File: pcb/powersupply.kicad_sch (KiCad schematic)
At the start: 33 parts, among them Q2 AO3401A, Q3 2N7002, Q9 AO3401A, U10 SMAJ16A-TR, U4 TPS54302, U5 SMAJ16A-TR, U6 AMS1117-3.3

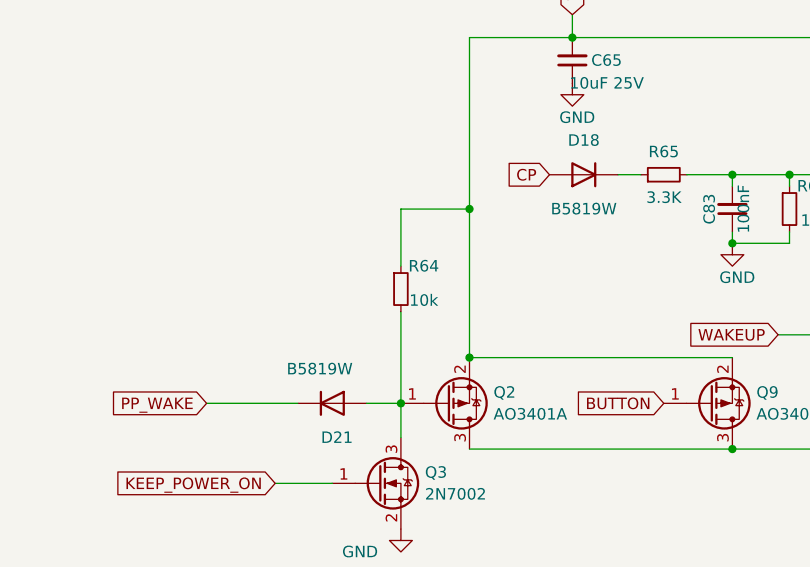
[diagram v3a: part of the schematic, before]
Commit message: Made PP standby and button pullup 1k Improved connection of TVS diode
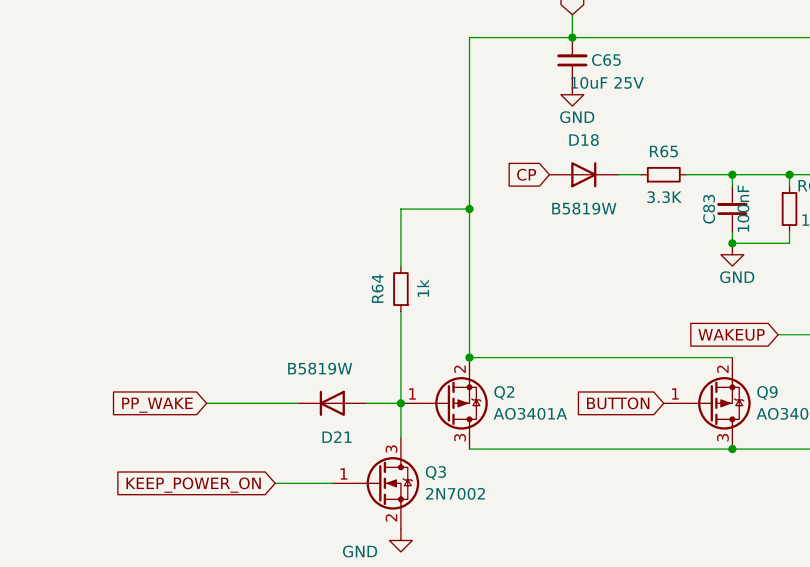
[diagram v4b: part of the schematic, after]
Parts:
- R64: value 10k -> 1k; LCSC C17414 -> C17513; LINK https://jlcpcb.com/partdetail/18102-0805W8F1002T5E/C17414 -> https://jlcpcb.com/partdetail/18201-0805W8F1001T5E/C17513
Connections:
- net 12V_P: now also R64.2; no longer R64.1
- net at D21.2 (A), Q2.1 (G), Q3.3 (D): now also R64.1; no longer R64.2
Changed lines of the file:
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@@
+    )
+  )
+  (symbol (lib_id "Device:R_Small") (at 109.22 72.39 180) (unit 1)
+    (in_bom yes) (on_board yes) (dnp no)
+    (property "Reference" "R64" (at 106.68 72.39 90)
+      (effects (font (size 1.27 1.27)))
+    )
+    (property "Value" "1k" (at 111.76 72.39 90)
+      (effects (font (size 1.27 1.27)))
+    )
+    (property "Footprint" "Resistor_SMD:R_0805_2012Metric_Pad1.20x1.40mm_HandSolder" (at 109.22 72.39 0)
+      (effects (font (size 1.27 1.27)) hide)
+    )
+    (property "Datasheet" "https://datasheet.lcsc.com/lcsc/1811101920_UNI-ROYAL-Uniroyal-Elec-0603WAF3301T5E_C22978.pdf" (at 109.22 72.39 0)
+      (effects (font (size 1.27 1.27)) hide)
+    )
+    (property "LCSC" "C17513" (at 109.22 72.39 90)
+      (effects (font (size 1.27 1.27)) hide)
+    )
+    (property "LINK" "https://jlcpcb.com/partdetail/18201-0805W8F1001T5E/C17513" (at 109.22 72.39 0)
+      (effects (font (size 1.27 1.27)) hide)
+    )
+    (pin "1")
+    (pin "2")
+    (instances
+      (project "qca7000"
+        (path "/e63e39d7-6ac0-4ffd-8aa3-1841a4541b55/81db238c-e53f-4d52-98ea-36a1df697651"
+          (reference "R64") (unit 1)
+        )
+      )
     )
   )
@@
         )
       )
-    )
-  )
-  (symbol (lib_id "Device:R_Small") (at 109.22 72.39 0) (unit 1)
-    (in_bom yes) (on_board yes) (dnp no)
-    (property "Reference" "R64" (at 111.76 69.85 0)
-      (effects (font (size 1.27 1.27)))
-    )
-    (property "Value" "10k" (at 111.76 73.66 0)
-      (effects (font (size 1.27 1.27)))
-    )
-    (property "Footprint" "Resistor_SMD:R_0805_2012Metric_Pad1.20x1.40mm_HandSolder" (at 109.22 72.39 0)
-      (effects (font (size 1.27 1.27)) hide)
-    )
-    (property "Datasheet" "~" (at 109.22 72.39 0)
-      (effects (font (size 1.27 1.27)) hide)
-    )
-    (property "LCSC" "C17414" (at 109.22 72.39 0)
-      (effects (font (size 1.27 1.27)) hide)
-    )
-    (property "LINK" "https://jlcpcb.com/partdetail/18102-0805W8F1002T5E/C17414" (at 109.22 72.39 0)
-      (effects (font (size 1.27 1.27)) hide)
-    )
-    (pin "1")
-    (pin "2")
-    (instances
-      (project "qca7000"
-        (path "/e63e39d7-6ac0-4ffd-8aa3-1841a4541b55/81db238c-e53f-4d52-98ea-36a1df697651"
-          (reference "R64") (unit 1)
-        )
-      )
